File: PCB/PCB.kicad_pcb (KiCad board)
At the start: 2 copper layers, 99.1 x 74.3 mm, 51 parts

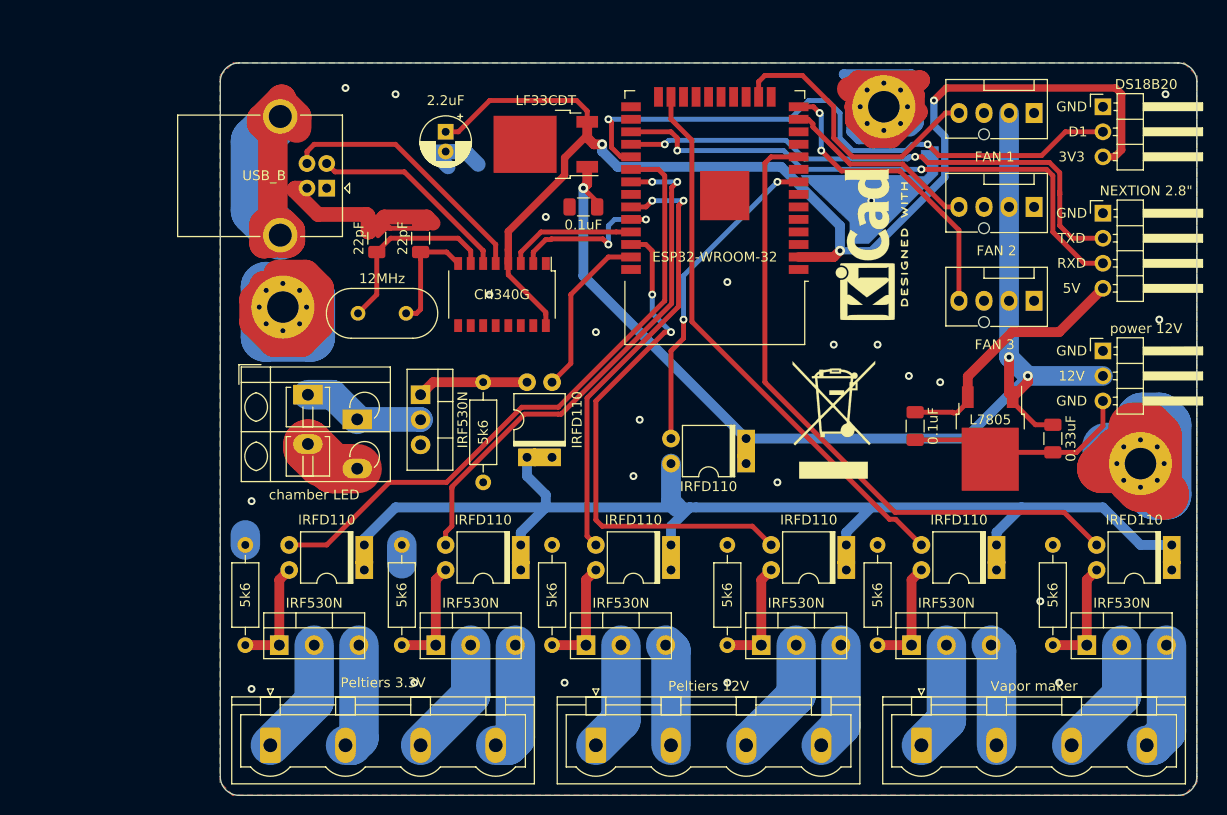
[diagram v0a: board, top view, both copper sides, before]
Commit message: PCB General UPGRADE
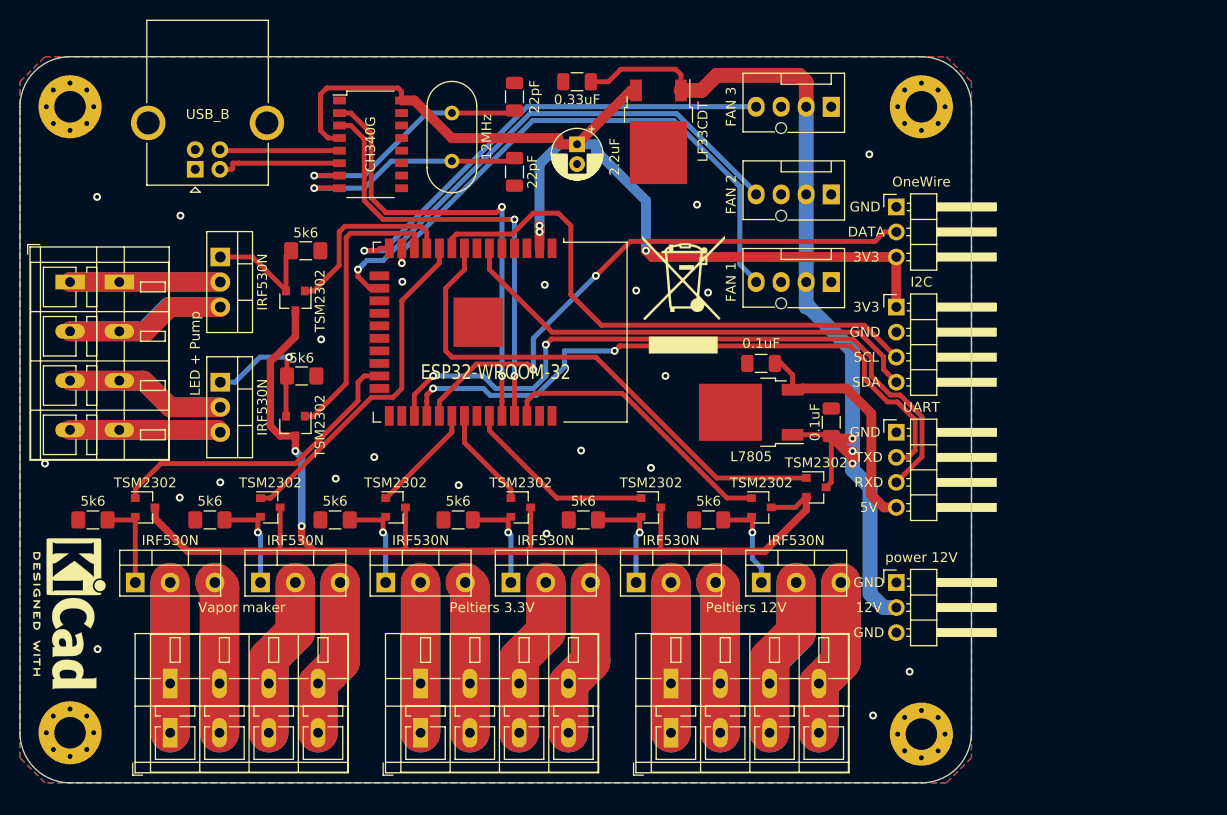
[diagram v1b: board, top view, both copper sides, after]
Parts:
- removed the 0.1uF at (202.6, 88.3)
- removed the 0.1uF at (168.9, 66.0)
- removed the 22pF at (152.4, 69.2)
- removed the 22pF at (148.0, 69.2)
- removed the 5k6 at (158.8, 83.8)
- removed the 5k6 at (216.5, 110.5)
- removed the 5k6 at (198.8, 110.5)
- removed the 5k6 at (150.5, 110.5)
- removed the 5k6 at (134.6, 110.5)
- removed the 5k6 at (183.5, 110.5)
- removed the 5k6 at (165.7, 110.5)
- removed DS18B20: , Connector_PinHeader_2.54mm:PinHeader_1x03_P2.54mm_Horizontal
- removed the IRF530N at (152.4, 85.1)
- removed the IRF530N at (221.0, 110.5)
- removed the IRF530N at (203.2, 110.5)
- removed the IRF530N at (154.9, 110.5)
- removed the IRF530N at (139.1, 110.5)
- removed the IRF530N at (188.0, 110.5)
- removed the IRF530N at (170.2, 110.5)
- removed IRFD110 (x8): , Package_DIP:Vishay_HVM-DIP-3_W7.62mm
- removed NEXTION 2.8": , Connector_PinHeader_2.54mm:PinHeader_1x04_P2.54mm_Horizontal
- removed the Peltiers 12V at (170.2, 120.7)
- removed the Peltiers 3.3V at (137.2, 120.7)
- removed the REF** at (138.4, 76.2)
- removed the REF** at (225.4, 92.1)
- removed the REF** at (199.4, 55.9)
- removed the Vapor maker at (203.2, 120.7)
- removed chamber LED: , TerminalBlock_WAGO:TerminalBlock_WAGO_804-102_1x02_P5.00mm_45Degree
- added 0.1uF: , Capacitor_SMD:C_1206_3216Metric, F.Cu at (186.9, 81.9)
- added 0.1uF: , Capacitor_SMD:C_1206_3216Metric, F.Cu at (194.1, 87.9)
- added 22pF: , Capacitor_SMD:C_1206_3216Metric, F.Cu at (161.9, 62.5)
- added 22pF: , Capacitor_SMD:C_1206_3216Metric, F.Cu at (161.9, 54.9)
- added 5k6: , Resistor_SMD:R_1206_3216Metric_Pad1.42x1.75mm_HandSolder, F.Cu at (140.3, 83.2)
- added 5k6: , Resistor_SMD:R_1206_3216Metric_Pad1.42x1.75mm_HandSolder, F.Cu at (140.8, 70.5)
- added 5k6: , Resistor_SMD:R_1206_3216Metric_Pad1.42x1.75mm_HandSolder, F.Cu at (131.0, 97.8)
- added 5k6: , Resistor_SMD:R_1206_3216Metric_Pad1.42x1.75mm_HandSolder, F.Cu at (119.2, 97.8)
- added 5k6: , Resistor_SMD:R_1206_3216Metric_Pad1.42x1.75mm_HandSolder, F.Cu at (156.2, 97.8)
- added 5k6: , Resistor_SMD:R_1206_3216Metric_Pad1.42x1.75mm_HandSolder, F.Cu at (143.7, 97.8)
- added 5k6: , Resistor_SMD:R_1206_3216Metric_Pad1.42x1.75mm_HandSolder, F.Cu at (181.6, 97.8)
- added 5k6: , Resistor_SMD:R_1206_3216Metric_Pad1.42x1.75mm_HandSolder, F.Cu at (168.9, 97.8)
- added H1: MountingHole_Pad, MountingHole:MountingHole_3.2mm_M3_Pad_Via, F.Cu at (203.2, 119.5)
- added H2: MountingHole_Pad, MountingHole:MountingHole_3.2mm_M3_Pad_Via, F.Cu at (116.8, 55.9)
- added H3: MountingHole_Pad, MountingHole:MountingHole_3.2mm_M3_Pad_Via, F.Cu at (203.2, 55.9)
- added H4: MountingHole_Pad, MountingHole:MountingHole_3.2mm_M3_Pad_Via, F.Cu at (116.8, 119.4)
- added I2C: , Connector_PinHeader_2.54mm:PinHeader_1x04_P2.54mm_Horizontal, F.Cu at (200.7, 76.2)
- added IRF530N: , Package_TO_SOT_THT:TO-220-3_Vertical, F.Cu at (132.1, 83.8)
- added IRF530N: , Package_TO_SOT_THT:TO-220-3_Vertical, F.Cu at (132.1, 71.1)
- added IRF530N: , Package_TO_SOT_THT:TO-220-3_Vertical, F.Cu at (137.2, 104.1)
- added IRF530N: , Package_TO_SOT_THT:TO-220-3_Vertical, F.Cu at (124.5, 104.1)
- added IRF530N: , Package_TO_SOT_THT:TO-220-3_Vertical, F.Cu at (162.6, 104.1)
- added IRF530N: , Package_TO_SOT_THT:TO-220-3_Vertical, F.Cu at (149.9, 104.1)
- added IRF530N: , Package_TO_SOT_THT:TO-220-3_Vertical, F.Cu at (188.0, 104.1)
- added IRF530N: , Package_TO_SOT_THT:TO-220-3_Vertical, F.Cu at (175.3, 104.1)
- added LED + Pump: , TerminalBlock_WAGO:TerminalBlock_WAGO_236-104_1x04_P5.00mm_45Degree, F.Cu at (116.8, 73.7)
- added OneWire: , Connector_PinHeader_2.54mm:PinHeader_1x03_P2.54mm_Horizontal, F.Cu at (200.7, 66.0)
- added Peltiers 12V: , TerminalBlock_WAGO:TerminalBlock_WAGO_236-104_1x04_P5.00mm_45Degree, F.Cu at (177.8, 119.4)
- added Peltiers 3.3V: , TerminalBlock_WAGO:TerminalBlock_WAGO_236-104_1x04_P5.00mm_45Degree, F.Cu at (152.4, 119.4)
- added TSM2302: , Package_TO_SOT_SMD:SOT-23, F.Cu at (139.7, 88.3)
- added TSM2302: , Package_TO_SOT_SMD:SOT-23, F.Cu at (139.7, 75.6)
- added TSM2302: , Package_TO_SOT_SMD:SOT-23, F.Cu at (137.2, 96.5)
- added TSM2302: , Package_TO_SOT_SMD:SOT-23, F.Cu at (124.5, 96.5)
- added TSM2302: , Package_TO_SOT_SMD:SOT-23, F.Cu at (162.6, 96.5)
- added TSM2302: , Package_TO_SOT_SMD:SOT-23, F.Cu at (149.9, 96.5)
- added TSM2302: , Package_TO_SOT_SMD:SOT-23, F.Cu at (187.0, 96.5)
- added TSM2302: , Package_TO_SOT_SMD:SOT-23, F.Cu at (175.8, 96.5)
- added TSM2302: , Package_TO_SOT_SMD:SOT-23, F.Cu at (192.5, 94.5)
- added UART: , Connector_PinHeader_2.54mm:PinHeader_1x04_P2.54mm_Horizontal, F.Cu at (200.7, 88.9)
- added Vapor maker: , TerminalBlock_WAGO:TerminalBlock_WAGO_236-104_1x04_P5.00mm_45Degree, F.Cu at (127.0, 119.4)
- moved REF** 88.3 mm to (117.5, 107.3), turned to 270 degrees
- moved REF** 82.1 mm to (126.4, 96.5), turned to 180 degrees
- moved 0.33uF 60.3 mm to (168.3, 53.3), turned to 180 degrees
- moved power 12V 31.5 mm to (200.7, 104.1)
- moved ESP32-WROOM-32 28.8 mm to (157.5, 78.7), turned to 270 degrees
- moved FAN 3 28.5 mm to (194.1, 55.9)
- moved FAN 1 26.8 mm to (194.1, 73.7)
- moved L7805 24.4 mm to (185.9, 86.9), turned to 180 degrees
- moved 12MHz 22.4 mm to (155.6, 56.5), turned to 270 degrees
- moved FAN 2 20.6 mm to (194.1, 64.8)
- moved REF** 20.3 mm to (159.4, 74.3), turned to 180 degrees
- moved CH340G 20.3 mm to (147.3, 59.7), turned to 0 degrees
- moved REF** 19.8 mm to (179.1, 74.9)
- moved USB_B 13.5 mm to (129.5, 62.2), turned to 90 degrees
- moved 2.2uF 13.4 mm to (168.3, 59.7)
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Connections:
- FAN 1 pad 4: Net-(J6-Pad4) -> Net-(J7-Pad4)
- FAN 2 pad 4: Net-(J7-Pad4) -> Net-(J6-Pad4)
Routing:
- net (no net): track 166.2 -> 0.00 mm
- net GND: track 117.2 -> 0.00 mm, vias 23 -> 22
- net Net-(Q10-Pad1) (its old number): track 115.2 -> 0.00 mm
- net Net-(Q10-Pad3): track 11.5 -> 122.2 mm, vias 0 -> 2
- net Net-(J12-Pad3): track 0.00 -> 57.3 mm
- net Net-(Q10-Pad1): track 64.7 -> 11.1 mm
- net Net-(J12-Pad4): track 0.00 -> 48.9 mm
- net Net-(Q11-Pad1): track 53.4 -> 10.3 mm, vias 2 -> 0
- net Net-(J7-Pad4): track 20.1 -> 55.6 mm, vias 0 -> 1
- net Net-(J11-Pad3): track 0.00 -> 32.7 mm
- net Net-(J11-Pad2): track 0.00 -> 32.6 mm
- net Net-(U1-Pad3): track 13.2 -> 45.3 mm, vias 0 -> 2
- net Net-(Q13-Pad1): track 66.4 -> 34.7 mm
- net Net-(J11-Pad4): track 0.00 -> 30.7 mm
- net Net-(Q15-Pad1): track 0.00 -> 29.0 mm
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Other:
- board size 99.1 x 74.3 mm -> 96.5 x 73.7 mm
- board text added: "CLOUD CHAMBER"
- board text added: "DATA"
- board text added: "SCL"
- board text added: "SDA"
- board text added: "Vilém Raška 2019"
- board text removed: "D1"
